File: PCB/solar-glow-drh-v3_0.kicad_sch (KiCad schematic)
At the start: 54 parts, among them J1 UPDI hdr, Q1 BCP5316MTWG, SW2 LED master, U1 AVR64DD28 (VQFN28), U2 ALD910025SALI, U3 LIS2DH12, U4 TLV431BCDBZR, U5 NT3H2211, U6 TPS22918

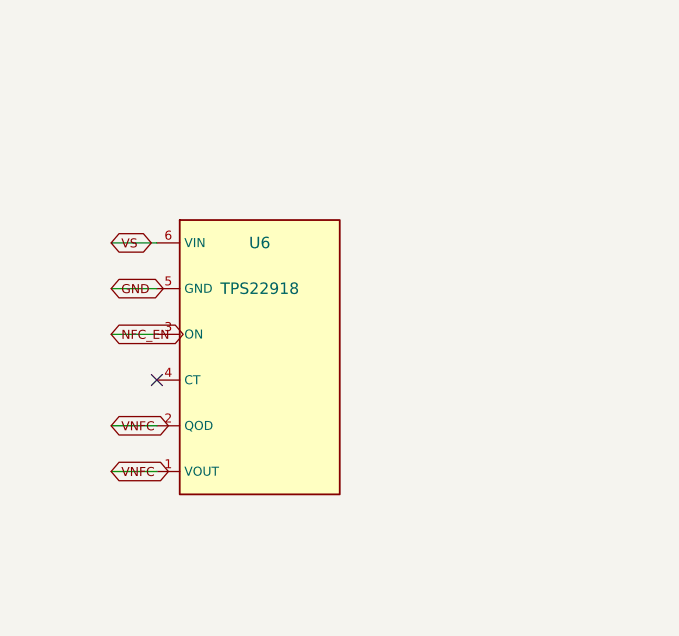
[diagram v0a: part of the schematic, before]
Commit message: Add files via upload
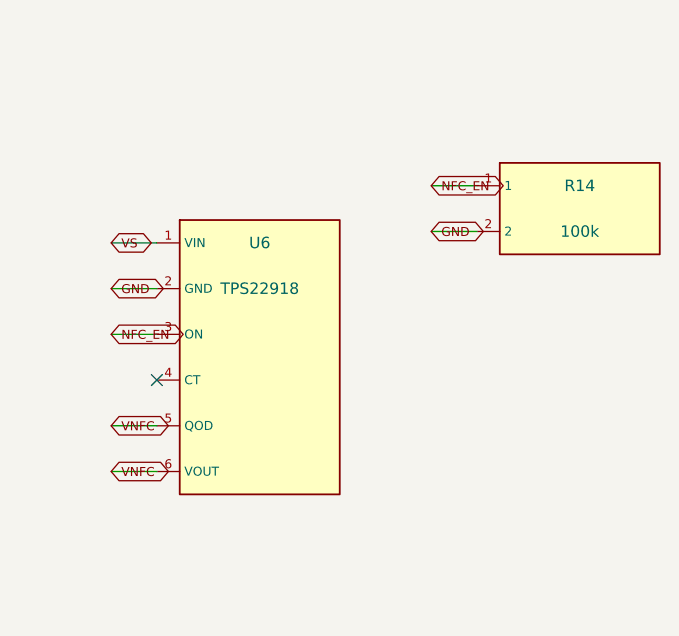
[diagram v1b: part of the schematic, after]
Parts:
- added R14: 100k, solarglow:R14, symbol solarglow:R14
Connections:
- net GND: now also U6.2 (GND), R14.2; no longer U6.5 (GND)
- net NFC_EN: now also R14.1
- net VNFC: now also U6.5 (QOD), U6.6 (VOUT); no longer U6.1 (VOUT), U6.2 (QOD)
- net VS: now also U6.1 (VIN); no longer U6.6 (VIN)
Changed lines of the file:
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@@
+	)
+	(symbol
+		(lib_id "solarglow:R14")
+		(at 685.8 69.85 0)
+		(unit 1)
+		(body_style 1)
+		(exclude_from_sim no)
+		(in_bom yes)
+		(on_board yes)
+		(in_pos_files yes)
+		(dnp no)
+		(property "Reference" "R14"
+			(at 697.23 69.85 0)
+			(show_name no)
+			(do_not_autoplace no)
+			(effects
+				(font
+					(size 1.27 1.27)
+				)
+			)
+		)
+		(property "Value" "100k"
+			(at 697.23 74.93 0)
+			(show_name no)
+			(do_not_autoplace no)
+			(effects
+				(font
+					(size 1.27 1.27)
+				)
+			)
+		)
+		(property "Footprint" "solarglow:R14"
+			(at 697.23 80.01 0)
+			(hide yes)
+			(show_name no)
+			(do_not_autoplace no)
+			(effects
+				(font
+					(size 1.27 1.27)
+				)
+			)
+		)
+		(property "Datasheet" ""
+			(at 685.8 69.85 0)
+			(hide yes)
+			(show_name no)
+			(do_not_autoplace no)
+			(effects
+				(font
+					(size 1.27 1.27)
+				)
+			)
+		)
+		(property "Description" ""
+			(at 685.8 69.85 0)
+			(hide yes)
+			(show_name no)
+			(do_not_autoplace no)
+			(effects
+				(font
+					(size 1.27 1.27)
+				)
+			)
+		)
+		(pin "1"
+		)
+		(pin "2"
+		)
+		(instances
+			(project "solar-glow-drh-v2_2"
+				(path "/bf17630f-b49b-49a7-9335-83fa0a7a44d0"
+					(reference "R14")
+					(unit 1)
+				)
+			)
+		)
 	)
 	(symbol
@@
 				)
 			)
+		)
+	)
+	(wire
+		(pts
+			(xy 685.8 69.85) (xy 680.72 69.85)
+		)
+		(stroke
+			(width 0)
+			(type default)
+		)
+	)
+	(wire
+		(pts
+			(xy 685.8 74.93) (xy 680.72 74.93)
+		)
+		(stroke
+			(width 0)
+			(type default)
+		)
+	)
+	(global_label "NFC_EN"
+		(shape bidirectional)
+		(at 680.72 69.85 0)
+		(effects
+			(font
+				(size 1 1)
+			)
+		)
+		(property "Intersheetrefs" "${INTERSHEET_REFS}"
+			(at 345.44 63.5 0)
+			(hide yes)
+			(show_name no)
+			(do_not_autoplace no)
+			(effects
+				(font
+					(size 1.27 1.27)
+				)
+			)
+		)
+	)
+	(global_label "GND"
+		(shape bidirectional)
+		(at 680.72 74.93 0)
+		(effects
+			(font
+				(size 1 1)
+			)
+		)
+		(property "Intersheetrefs" "${INTERSHEET_REFS}"
+			(at 345.44 63.5 0)
+			(hide yes)
+			(show_name no)
+			(do_not_autoplace no)
+			(effects
+				(font
+					(size 1.27 1.27)
+				)
+			)

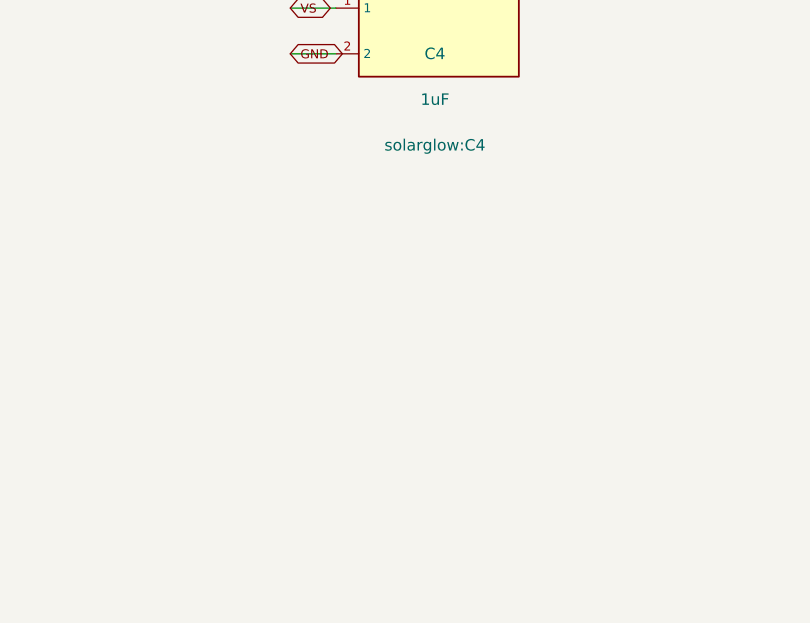
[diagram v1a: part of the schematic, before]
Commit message: Add files via upload
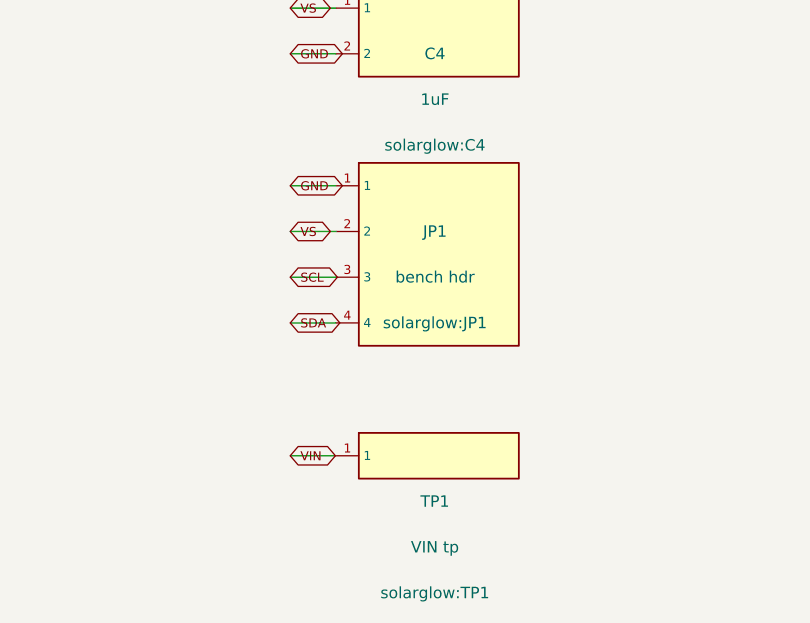
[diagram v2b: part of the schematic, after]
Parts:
- added JP1: bench hdr, solarglow:JP1, symbol solarglow:JP1
- added TP1: VIN tp, solarglow:TP1, symbol solarglow:TP1
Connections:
- net GND: now also JP1.1
- net SCL: now also JP1.3
- net SDA: now also JP1.4
- net VIN: now also TP1.1
- net VS: now also JP1.2

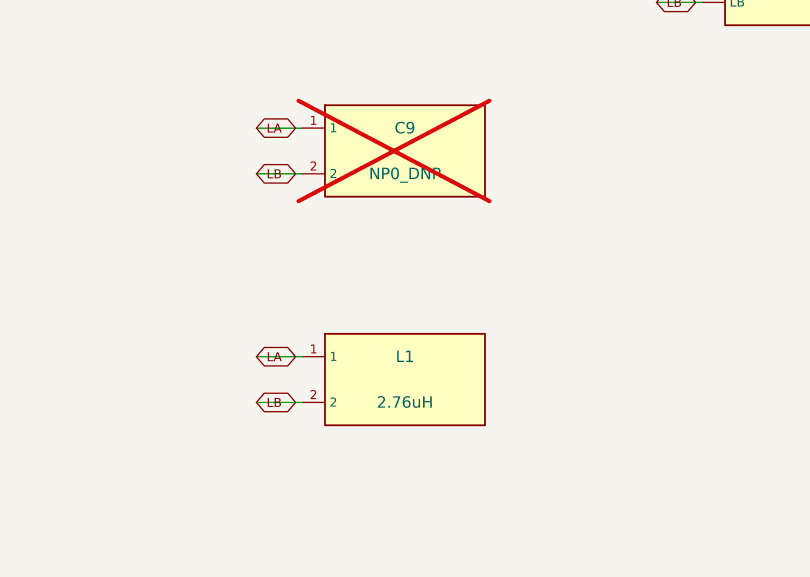
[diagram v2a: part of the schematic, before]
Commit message: Add files via upload
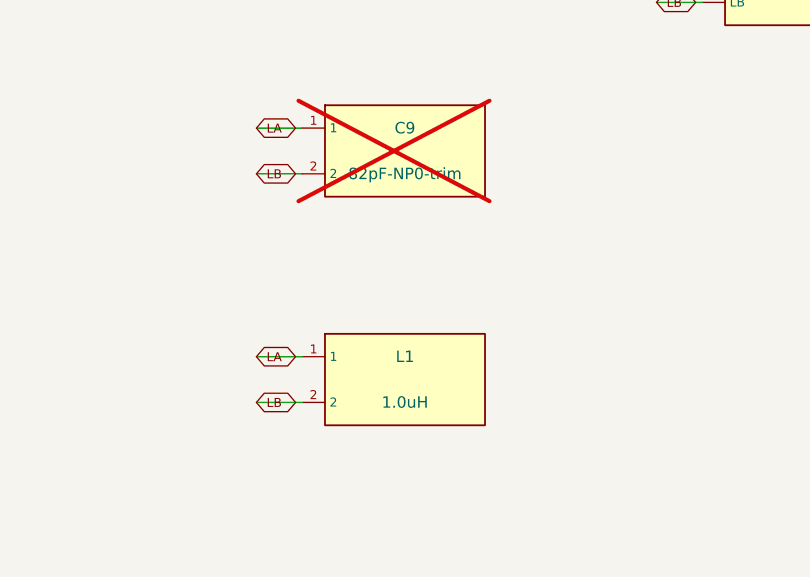
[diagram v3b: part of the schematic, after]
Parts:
- C9: value NP0_DNP -> 82pF-NP0-trim
- L1: value 2.76uH -> 1.0uH
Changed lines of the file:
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@@
 			)
 		)
-		(property "Value" "2.76uH"
+		(property "Value" "1.0uH"
 			(at 571.5 149.86 0)
 			(show_name no)
@@
 			)
 		)
-		(property "Value" "NP0_DNP"
+		(property "Value" "82pF-NP0-trim"
 			(at 571.5 124.46 0)
 			(show_name no)

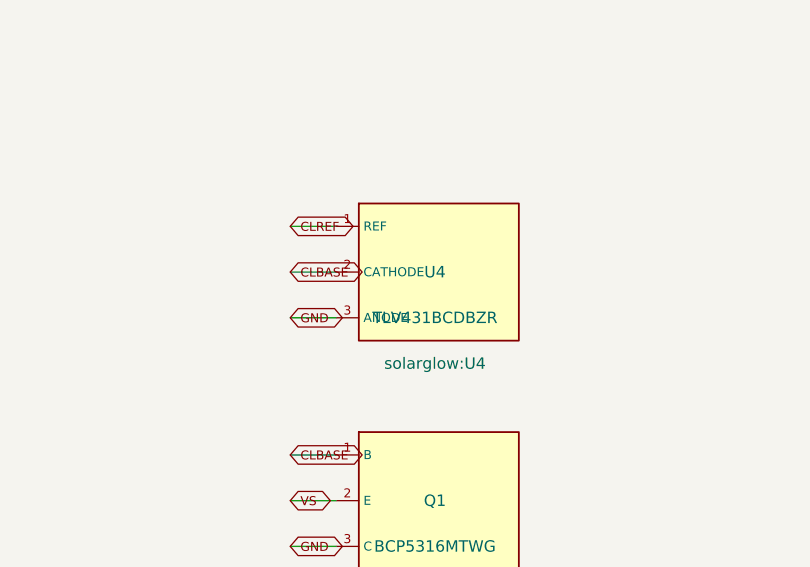
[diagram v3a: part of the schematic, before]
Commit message: Add files via upload
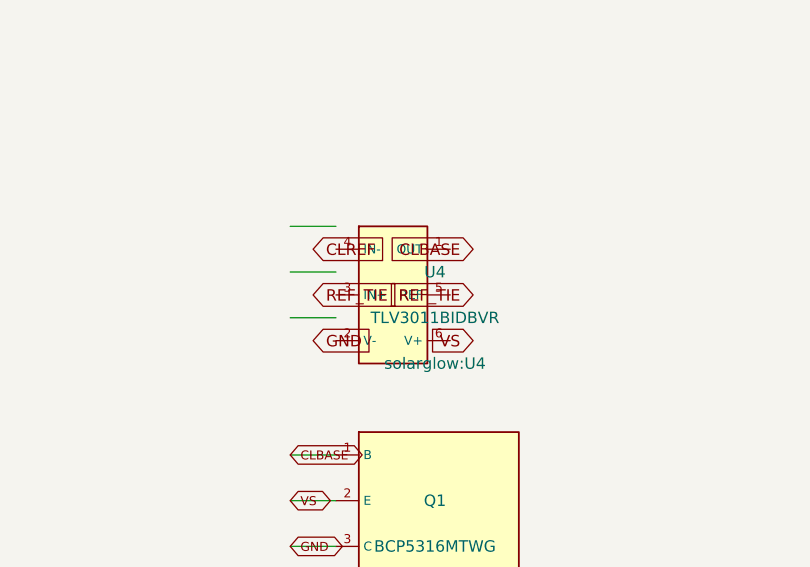
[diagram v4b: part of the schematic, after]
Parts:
- U4: value TLV431BCDBZR -> TLV3011BIDBVR
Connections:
- net CLBASE: no longer U4.2 (CATHODE)
- net CLREF: no longer U4.1 (REF)
- net GND: no longer U4.3 (ANODE)
